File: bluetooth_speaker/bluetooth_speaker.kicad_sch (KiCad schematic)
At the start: 23 parts, among them J1 Conn_Coaxial, J2 USB_C_Receptacle_USB2.0_16P, J3 282836-4, J5 Conn_01x04_Pin, U4 ESP32-D0WD-V3, Y1 40MHz(±10 ppm)

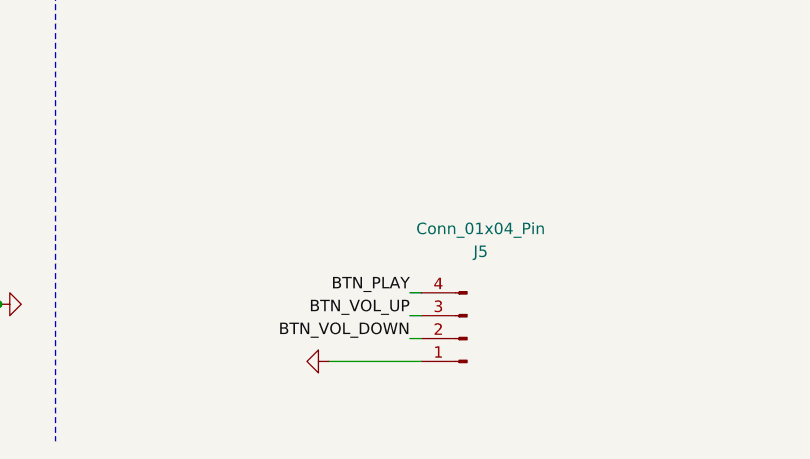
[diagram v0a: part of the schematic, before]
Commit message: again
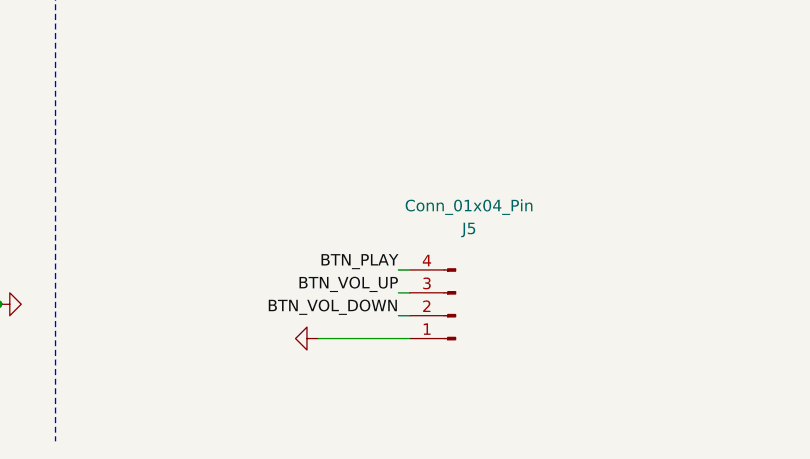
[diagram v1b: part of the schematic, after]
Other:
- moved on the sheet: J5
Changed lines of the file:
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@@
 	(wire
 		(pts
-			(xy 137.16 187.96) (xy 147.32 187.96)
+			(xy 135.89 185.42) (xy 146.05 185.42)
 		)
 		(stroke
@@
 	(wire
 		(pts
-			(xy 146.05 185.42) (xy 147.32 185.42)
+			(xy 144.78 182.88) (xy 146.05 182.88)
 		)
 		(stroke
@@
 	(wire
 		(pts
-			(xy 146.05 182.88) (xy 147.32 182.88)
+			(xy 144.78 180.34) (xy 146.05 180.34)
 		)
 		(stroke
@@
 	(wire
 		(pts
-			(xy 146.05 180.34) (xy 147.32 180.34)
+			(xy 144.78 177.8) (xy 146.05 177.8)
 		)
 		(stroke
@@
 	)
 	(label "BTN_VOL_UP"
-		(at 146.05 182.88 180)
+		(at 144.78 180.34 180)
 		(effects
 			(font
@@
 	)
 	(label "BTN_PLAY"
-		(at 146.05 180.34 180)
+		(at 144.78 177.8 180)
 		(effects
 			(font
@@
 	)
 	(label "BTN_VOL_DOWN"
-		(at 146.05 185.42 180)
+		(at 144.78 182.88 180)
 		(effects
 			(font
@@
 	(symbol
 		(lib_id "power:GND")
-		(at 137.16 187.96 270)
+		(at 135.89 185.42 270)
 		(unit 1)
 		(exclude_from_sim no)
@@
 		(fields_autoplaced yes)
 		(property "Reference" "#PWR047"
-			(at 130.81 187.96 0)
+			(at 129.54 185.42 0)
 			(effects
 				(font
@@
 		)
 		(property "Value" "GND"
-			(at 132.08 187.96 0)
+			(at 130.81 185.42 0)
 			(effects
 				(font
@@
 		)
 		(property "Footprint" ""
-			(at 137.16 187.96 0)
+			(at 135.89 185.42 0)
 			(effects
 				(font
@@
 		)
 		(property "Datasheet" ""
-			(at 137.16 187.96 0)
+			(at 135.89 185.42 0)
 			(effects
 				(font
@@
 		)
 		(property "Description" "Power symbol creates a global label with name \"GND\" , ground"
-			(at 137.16 187.96 0)
+			(at 135.89 185.42 0)
 			(effects
 				(font
@@
 	(symbol
 		(lib_id "Connector:Conn_01x04_Pin")
-		(at 152.4 185.42 180)
+		(at 151.13 182.88 180)
 		(unit 1)
 		(exclude_from_sim no)
@@
 		(dnp no)
 		(property "Reference" "J5"
-			(at 153.924 175.768 0)
+			(at 152.654 173.228 0)
 			(effects
 				(font
@@
 		)
 		(property "Value" "Conn_01x04_Pin"
-			(at 153.924 173.228 0)
+			(at 152.654 170.688 0)
 			(effects
 				(font
@@
 		)
 		(property "Footprint" "Connector_JST:JST_PH_B4B-PH-K_1x04_P2.00mm_Vertical"
-			(at 152.4 185.42 0)
+			(at 151.13 182.88 0)
 			(effects
 				(font
@@
 		)
 		(property "Datasheet" "~"
-			(at 152.4 185.42 0)
+			(at 151.13 182.88 0)
 			(effects
 				(font
@@
 		)
 		(property "Description" "Generic connector, single row, 01x04, script generated"
-			(at 152.4 185.42 0)
+			(at 151.13 182.88 0)
 			(effects
 				(font
